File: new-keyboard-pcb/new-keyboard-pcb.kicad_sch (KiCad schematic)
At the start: 0 parts

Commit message: schematic done
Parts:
- added C1, C2: 22pF, Capacitor_SMD:C_0805_2012Metric_Pad1.18x1.45mm_HandSolder, symbol Device:C_Small
- added C3: 1µF, Capacitor_SMD:C_0805_2012Metric_Pad1.18x1.45mm_HandSolder, symbol Device:C_Small
- added C4, C5, C6, C7: 0.1µF, Capacitor_SMD:C_0805_2012Metric_Pad1.18x1.45mm_HandSolder, symbol Device:C_Small
- added CH1, CH2, CH3, CH4: choc_v1_SW_HS, Kailh_PG1353_Hotswap:Kailh-PG1353-Hotswap-1U, symbol PCM_marbastlib-choc:choc_v1_SW_HS_CPG135001S30
- added D1, D2, D3, D4: D_Small, Diode_SMD:D_SOD-123, symbol Device:D_Small
- added F1: 500mA, Fuse:Fuse_1206_3216Metric_Pad1.42x1.75mm_HandSolder, symbol Device:Polyfuse_Small
- added R1, R4: 10k, Resistor_SMD:R_0805_2012Metric_Pad1.20x1.40mm_HandSolder, symbol Device:R_Small
- added R2, R3: 22, Resistor_SMD:R_0805_2012Metric_Pad1.20x1.40mm_HandSolder, symbol Device:R_Small
- added SW1: SW_Push, random-keyboard-parts.pretty-master:SKQG-1155865, symbol Switch:SW_Push
- added U1: ATmega32U4-A, Package_QFP:TQFP-44_10x10mm_P0.8mm, symbol MCU_Microchip_ATmega:ATmega32U4-A
- added USB1: Molex-0548190589, random-keyboard-parts.pretty-master:Molex-0548190589, symbol random-keyboard-parts:Molex-0548190589
- added Y1: 16MHz, Crystal:Crystal_SMD_3225-4Pin_3.2x2.5mm_HandSoldering, symbol Device:Crystal_GND24_Small
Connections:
- new net: R1.2, SW1.2, U1.13 (~{RESET})
- new net: C2.2, U1.16 (XTAL2), Y1.3
- new net: C1.2, U1.17 (XTAL1), Y1.1
- new net: R3.2, U1.3 (D-)
- new net: R4.1, U1.33 (~{HWB}/PE2)
- new net: R2.2, U1.4 (D+)
- new net: C3.2, U1.6 (UCAP)
- new net: CH1.2, D1.2 (A)
- new net: CH3.2, D3.2 (A)
- new net: CH2.2, D2.2 (A)
- new net: CH4.2, D4.2 (A)
- new net +5V: C4.1, C5.1, C6.1, C7.1, F1.2, R1.1, U1.14 (VCC), U1.2 (UVCC), U1.24 (AVCC), U1.34 (VCC), U1.44 (AVCC), U1.7 (VBUS)
- new net COL0: CH1.1, CH3.1, U1.28 (PB4)
- new net COL1: CH2.1, CH4.1, U1.29 (PB5)
- new net D+: R2.1, USB1.3 (D+)
- new net D-: R3.1, USB1.4 (D-)
- new net GND: C1.1, C2.1, C3.1, C4.2, C5.2, C6.2, C7.2, R4.2, SW1.1, U1.15 (GND), U1.23 (GND), U1.35 (GND), U1.43 (GND), U1.5 (UGND), USB1.1 (GND), Y1.2, Y1.4
- new net ROW0: D1.1 (K), D2.1 (K), U1.27 (PD7)
- new net ROW1: D3.1 (K), D4.1 (K), U1.30 (PB6)
- new net VCC: F1.1, USB1.6 (SHIELD)

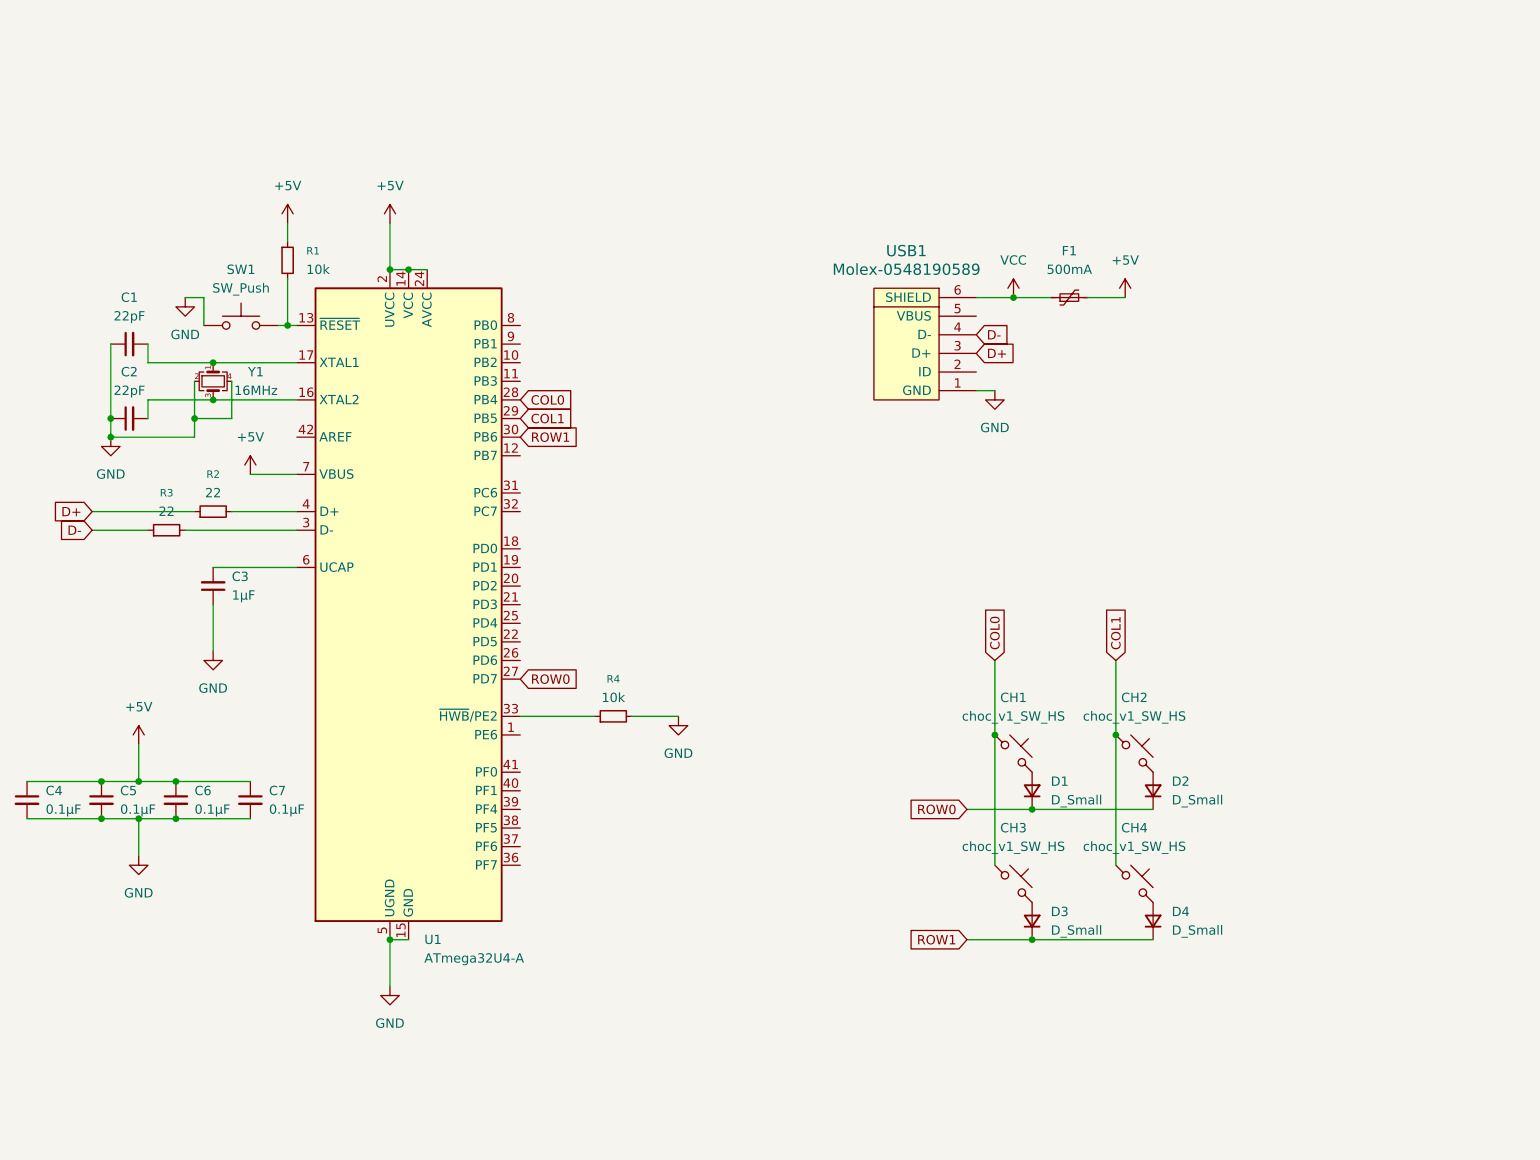
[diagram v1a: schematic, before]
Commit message: return to masterzen
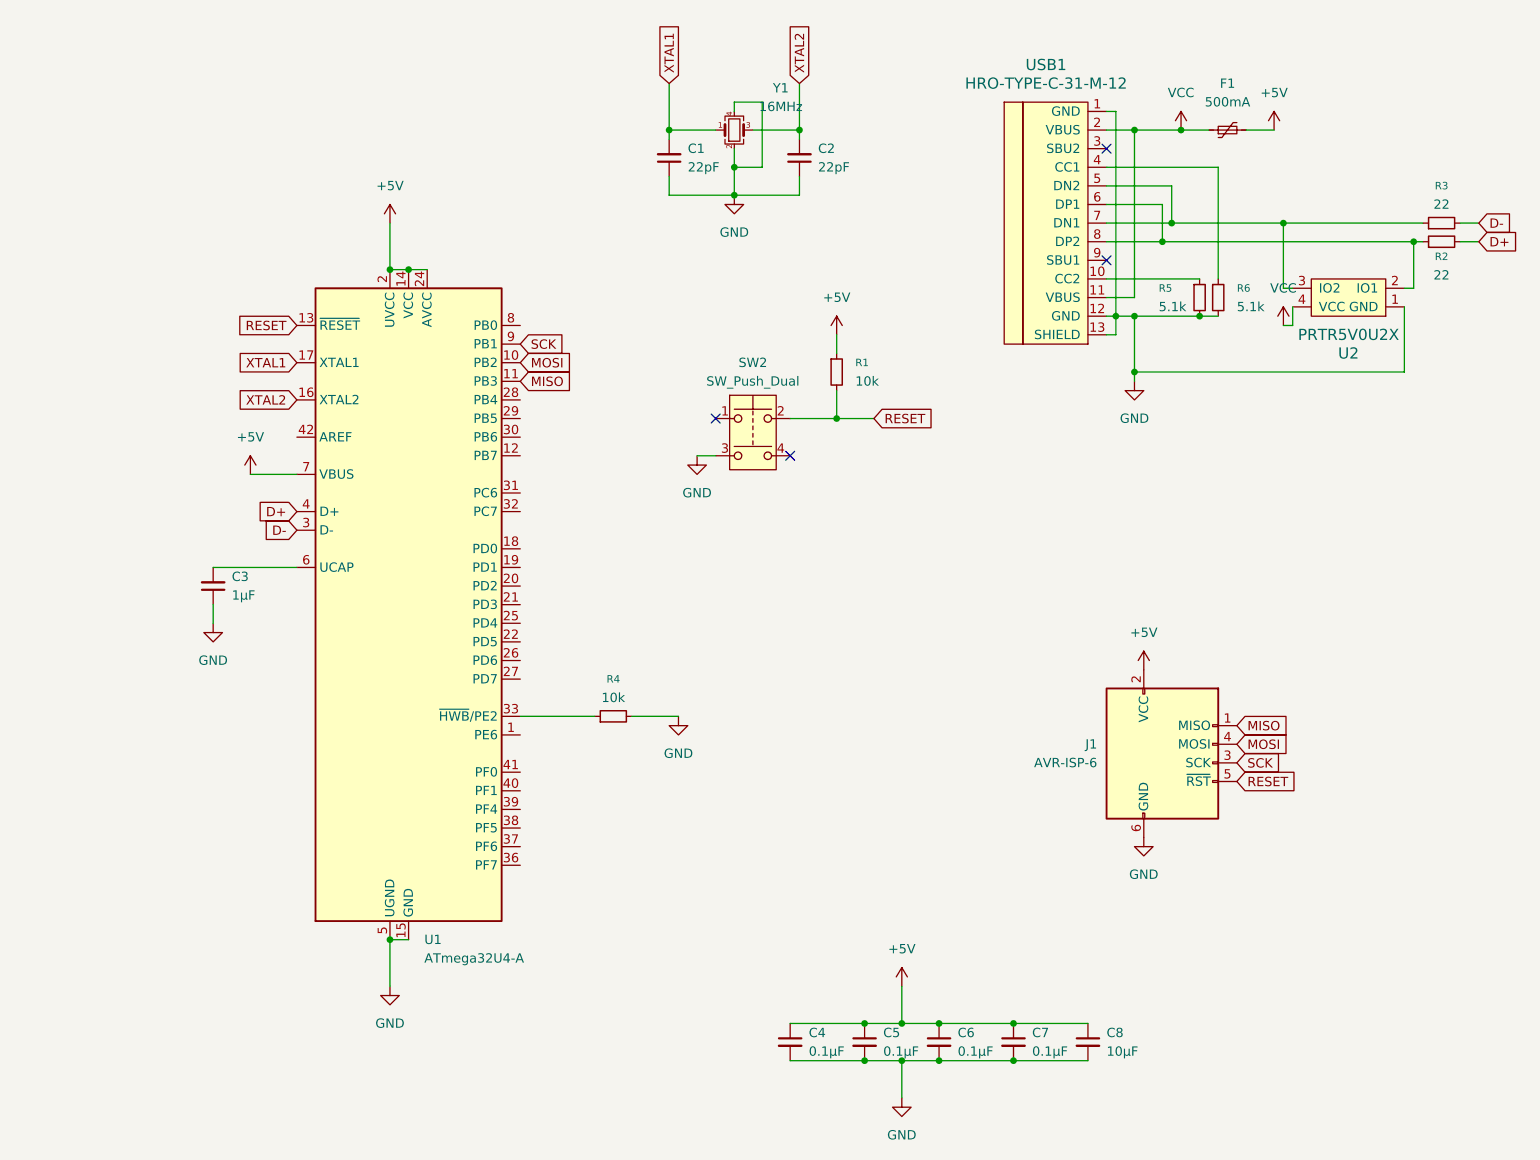
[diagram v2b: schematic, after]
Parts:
- removed CH1, CH2, CH3, CH4: choc_v1_SW_HS, Kailh_PG1353_Hotswap:Kailh-PG1353-Hotswap-1U, symbol PCM_marbastlib-choc:choc_v1_SW_HS_CPG135001S30
- removed D1, D2, D3, D4: D_Small, Diode_SMD:D_SOD-123, symbol Device:D_Small
- removed SW1: SW_Push, random-keyboard-parts.pretty-master:SKQG-1155865, symbol Switch:SW_Push
- removed USB1: Molex-0548190589, random-keyboard-parts.pretty-master:Molex-0548190589, symbol random-keyboard-parts:Molex-0548190589
- added C8: 10µF, Capacitor_SMD:C_0805_2012Metric_Pad1.18x1.45mm_HandSolder, symbol Device:C_Small
- added J1: AVR-ISP-6, symbol Connector:AVR-ISP-6
- added R5, R6: 5.1k, Resistor_SMD:R_0805_2012Metric_Pad1.20x1.40mm_HandSolder, symbol Device:R_Small
- added SW2: SW_Push_Dual, random-keyboard-parts.pretty-master:SKQG-1155865, symbol Switch:SW_Push_Dual
- added U2: PRTR5V0U2X, symbol random-keyboard-parts:PRTR5V0U2X
- added USB1: HRO-TYPE-C-31-M-12, symbol Type-C:HRO-TYPE-C-31-M-12
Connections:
- net +5V: now also C8.1, J1.2 (VCC)
- net D+: now also R2.2, U1.4 (D+); no longer R2.1
- net D-: now also R3.2, U1.3 (D-); no longer R3.1
- net GND: now also C8.2, J1.6 (GND), R5.2, R6.2, SW2.3, U2.1 (GND), USB1.1 (GND), USB1.12 (GND), USB1.13 (SHIELD)
- net VCC: now also U2.4 (VCC), USB1.11 (VBUS), USB1.2 (VBUS)
- net MOSI: now reaches U1.10 (PB2)
- net MOSI: now also J1.4 (MOSI)
- net MISO: now reaches U1.11 (PB3)
- net MISO: now also J1.1 (MISO)
- net RESET: now reaches R1.2, U1.13 (~{RESET})
- net RESET: now also J1.5 (~{RST}), SW2.2
- net XTAL2: now reaches C2.2, U1.16 (XTAL2), Y1.3
- net XTAL1: now reaches C1.2, U1.17 (XTAL1), Y1.1
- net SCK: now reaches U1.9 (PB1)
- net SCK: now also J1.3 (SCK)
- net COL0: no longer names the net of U1.28 (PB4)
- net COL1: no longer names the net of U1.29 (PB5)
- net ROW0: no longer names the net of U1.27 (PD7)
- net ROW1: no longer names the net of U1.30 (PB6)
- new net: R2.1, U2.2 (IO1), USB1.6 (DP1), USB1.8 (DP2)
- new net: R3.1, U2.3 (IO2), USB1.5 (DN2), USB1.7 (DN1)
- new net: R5.1, USB1.10 (CC2)
- new net: R6.1, USB1.4 (CC1)
- no-connect marks 0 -> 4
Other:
- moved on the sheet: C1, C2, C4, C5, C6, C7, F1, R1, Y1
